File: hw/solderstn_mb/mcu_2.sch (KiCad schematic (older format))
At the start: 4 parts

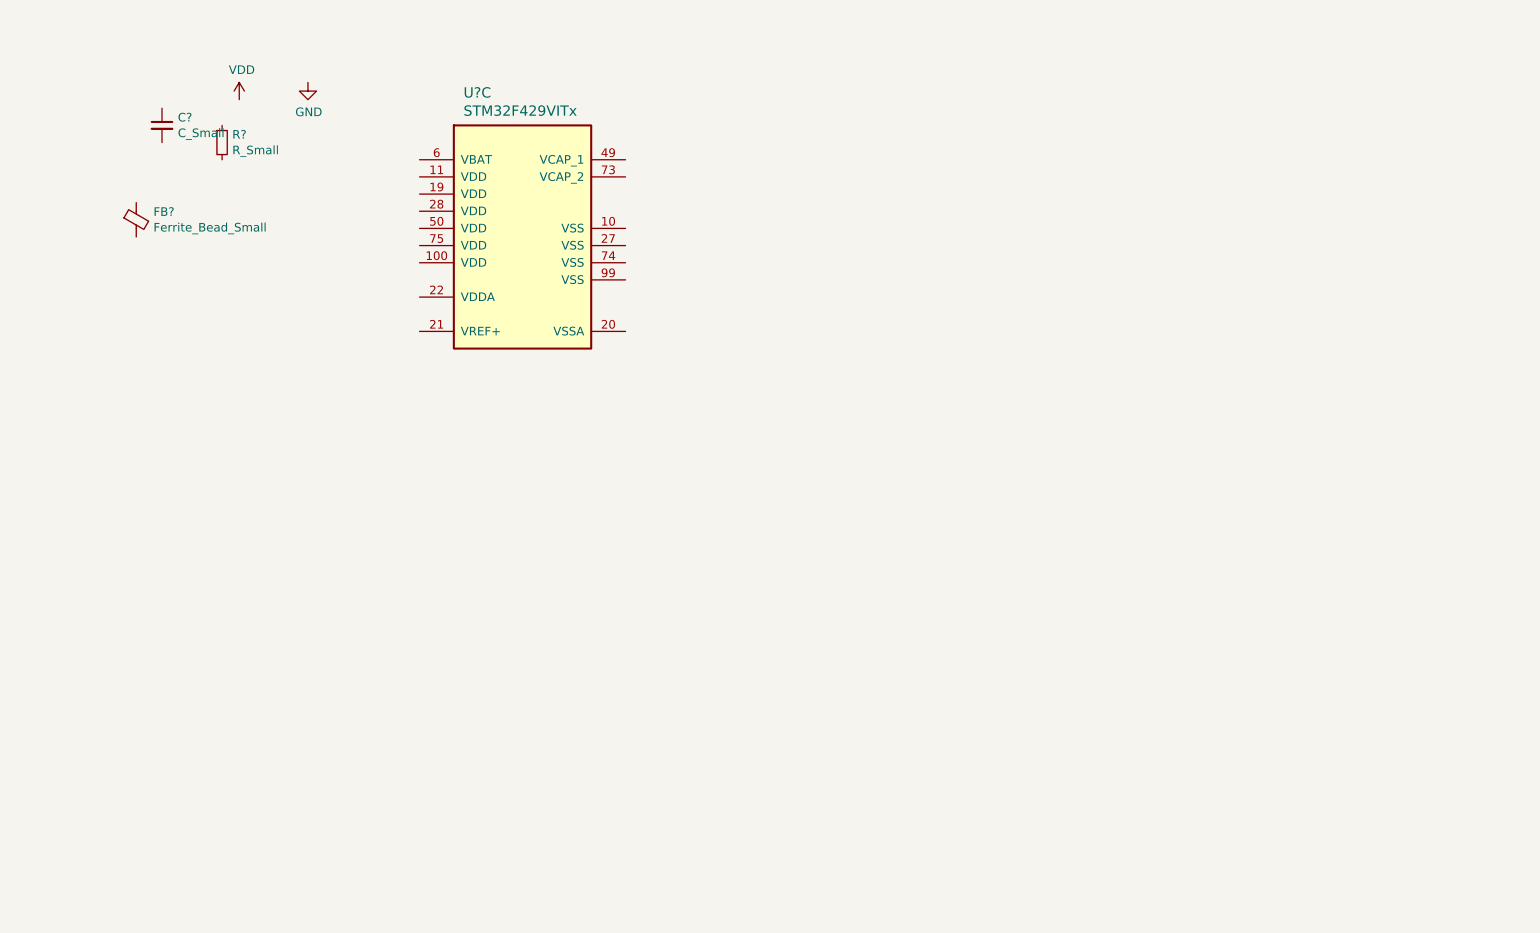
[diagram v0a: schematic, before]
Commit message: Summer vacation 2020 updates: * Front panel design rev 1 complete (incl Experimental outer board with optional linear touch sensors) * MB schematics AlmostDone(tm) - 'old' pinout supporting only one Rotary encoder * Lots of docs for new stuff
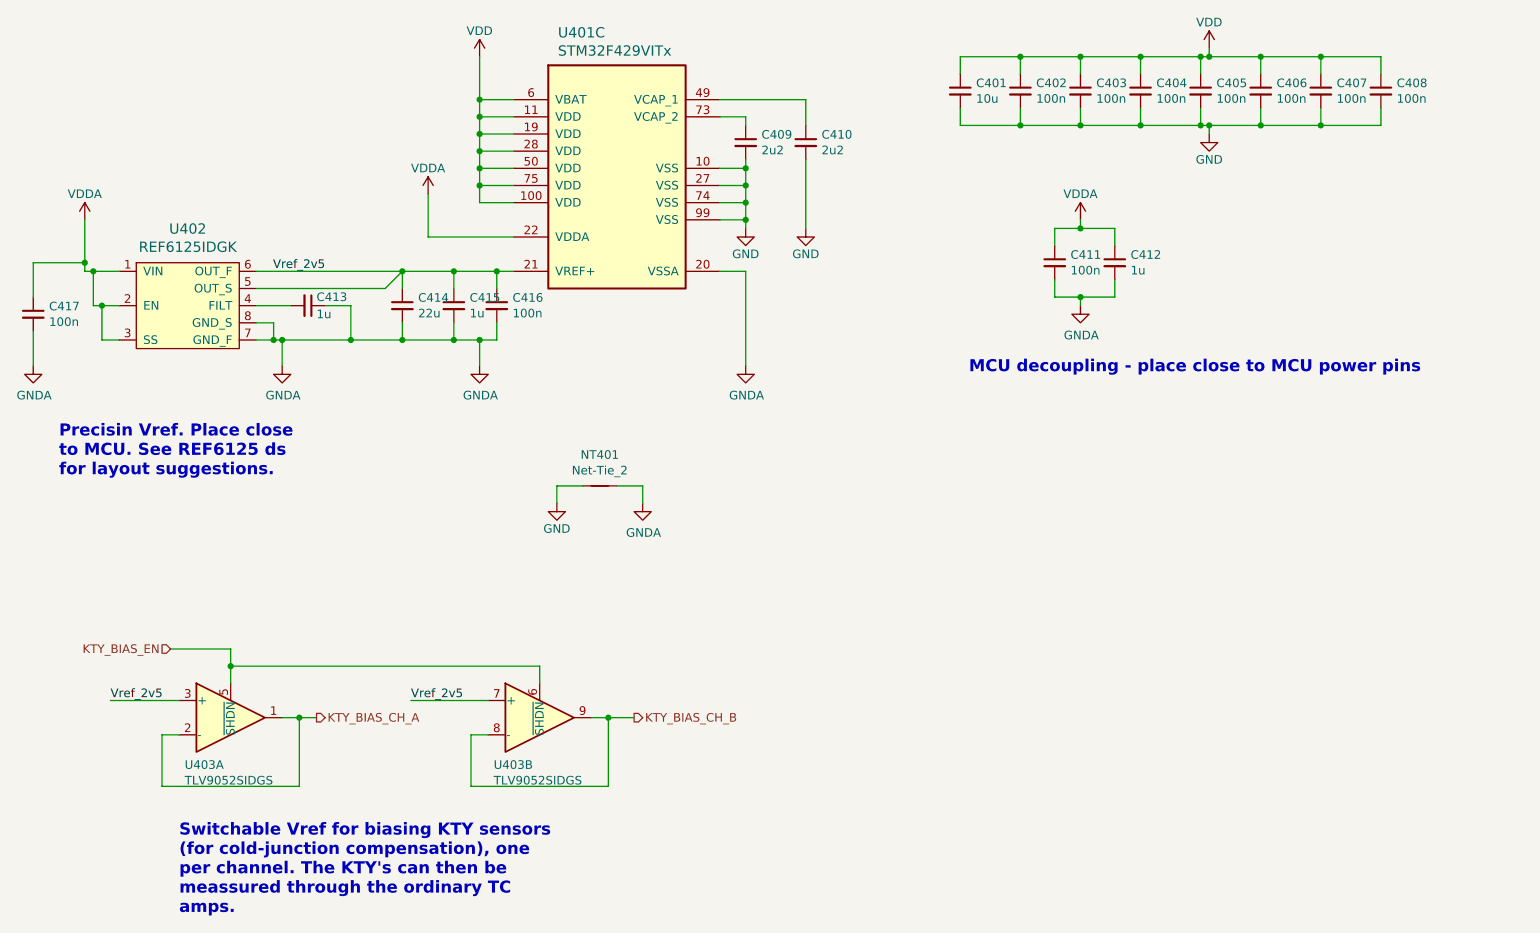
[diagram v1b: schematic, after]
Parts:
- removed C?: C_Small, symbol Device:C_Small
- removed FB?: Ferrite_Bead_Small, symbol customlib_mj:Ferrite_Bead_Small
- removed R?: R_Small, symbol Device:R_Small
- added C401: 10u, symbol Device:C_Small
- added C402, C403, C404, C405, C406, C407, C408, C411, C416, C417: 100n, symbol Device:C_Small
- added C409, C410: 2u2, symbol Device:C_Small
- added C412, C413, C415: 1u, symbol Device:C_Small
- added C414: 22u, symbol Device:C_Small
- added NT401: Net-Tie_2, symbol Device:Net-Tie_2
- added U402: REF6125IDGK, Package_SO:VSSOP-8_3.0x3.0mm_P0.65mm, symbol customlib_mj:REF6125IDGK
- added U403: TLV9052SIDGS, Package_SO:VSSOP-10_3x3mm_P0.5mm, symbol customlib_mj:TLV9052SIDGS
- gave numbers to parts that had none: 1
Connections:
- net GND: now also U401.10 (VSS), U401.27 (VSS), U401.74 (VSS), U401.99 (VSS), C401.2, C402.2, C403.2, C404.2, C405.2, C406.2, C407.2, C408.2, C409.2, C410.2, NT401.1
- net VDD: now also U401.100 (VDD), U401.11 (VDD), U401.19 (VDD), U401.28 (VDD), U401.50 (VDD), U401.6 (VBAT), U401.75 (VDD), C401.1, C402.1, C403.1, C404.1, C405.1, C406.1, C407.1, C408.1
- net GNDA: now reaches U401.20 (VSSA)
- net GNDA: now also C411.2, C412.2, C413.1, C414.2, C415.2, C416.2, C417.2, NT401.2, U402.7 (GND_F), U402.8 (GND_S)
- net Vref_2v5: now reaches U401.21 (VREF+)
- net Vref_2v5: now also C414.1, C415.1, C416.1, U402.5 (OUT_S), U402.6 (OUT_F), U403.3 (+), U403.7 (+)
- net VDDA: now reaches U401.22 (VDDA)
- net VDDA: now also C411.1, C412.1, C417.1, U402.1 (VIN), U402.2 (EN), U402.3 (SS)
- net at U401.49 (VCAP_1): now also C410.1
- net at U401.73 (VCAP_2): now also C409.1
- new net: C413.2, U402.4 (FILT)
- new net KTY_BIAS_CH_A: U403.1, U403.2 (-)
- new net KTY_BIAS_CH_B: U403.8 (-), U403.9
- new net KTY_BIAS_EN: U403.5 (~SHDN~), U403.6 (~SHDN~)
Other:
- note added: "MCU decoupling - place close to MCU power pins"
- note added: "Precisin Vref. Place close\nto MCU. See REF6125 ds\nfor layout suggestions."
- note added: "Switchable Vref for biasing KTY sensors\n(for cold-junction compensation), one\nper channel. The KTY's can then be\nmeassured through the ordinary TC \namps.\n"
- moved on the sheet: U401C
